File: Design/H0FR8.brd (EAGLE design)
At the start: 34.6 x 30 mm, 45 parts, among them P1 HEXABIT_17.32_NO_P6, Q1 MMBT3904LT1, U1 STM32G0B1CEU6N, U2 T2035H-6GD2PAK_T2550_STM-M, U3 VOT8121AM-VT, U4 TLP184_GR-TPL,SE, X1 XTALL_CSTCE8M00G52

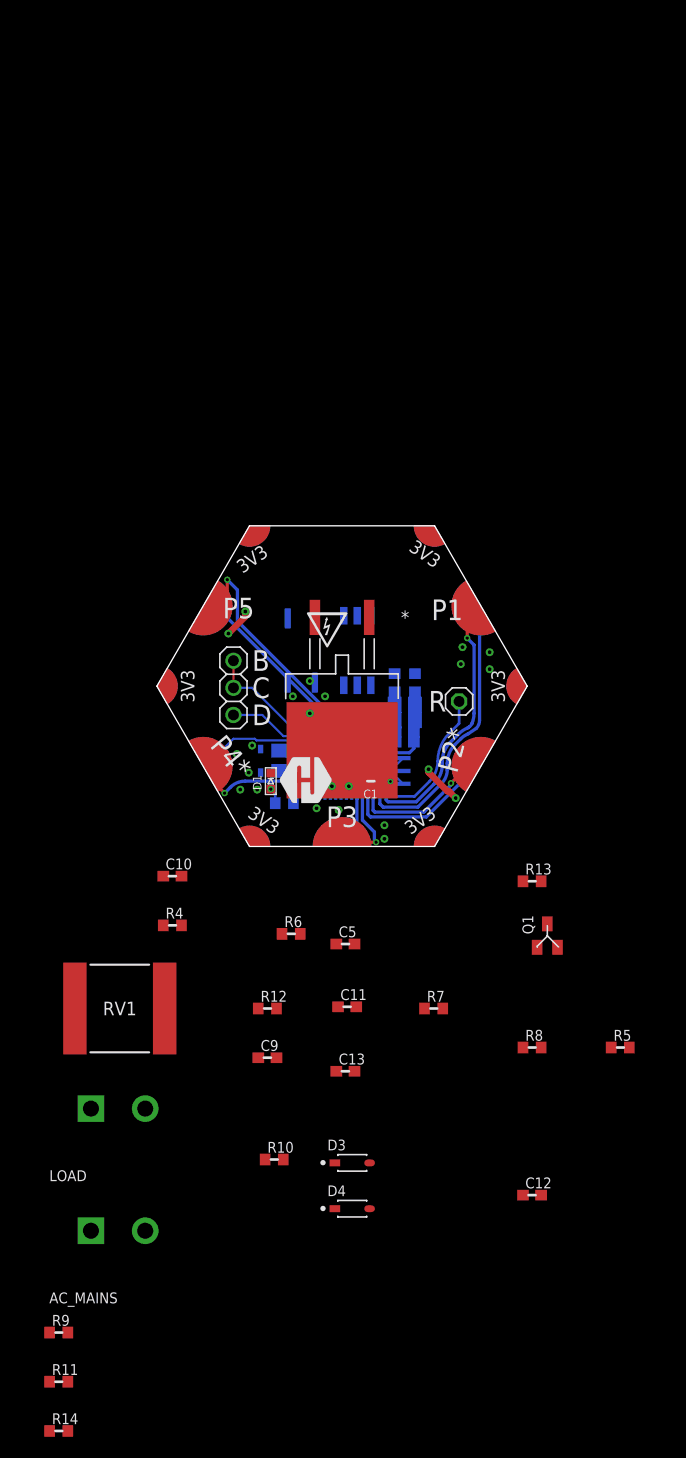
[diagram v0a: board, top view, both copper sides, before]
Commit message: Schematic modification
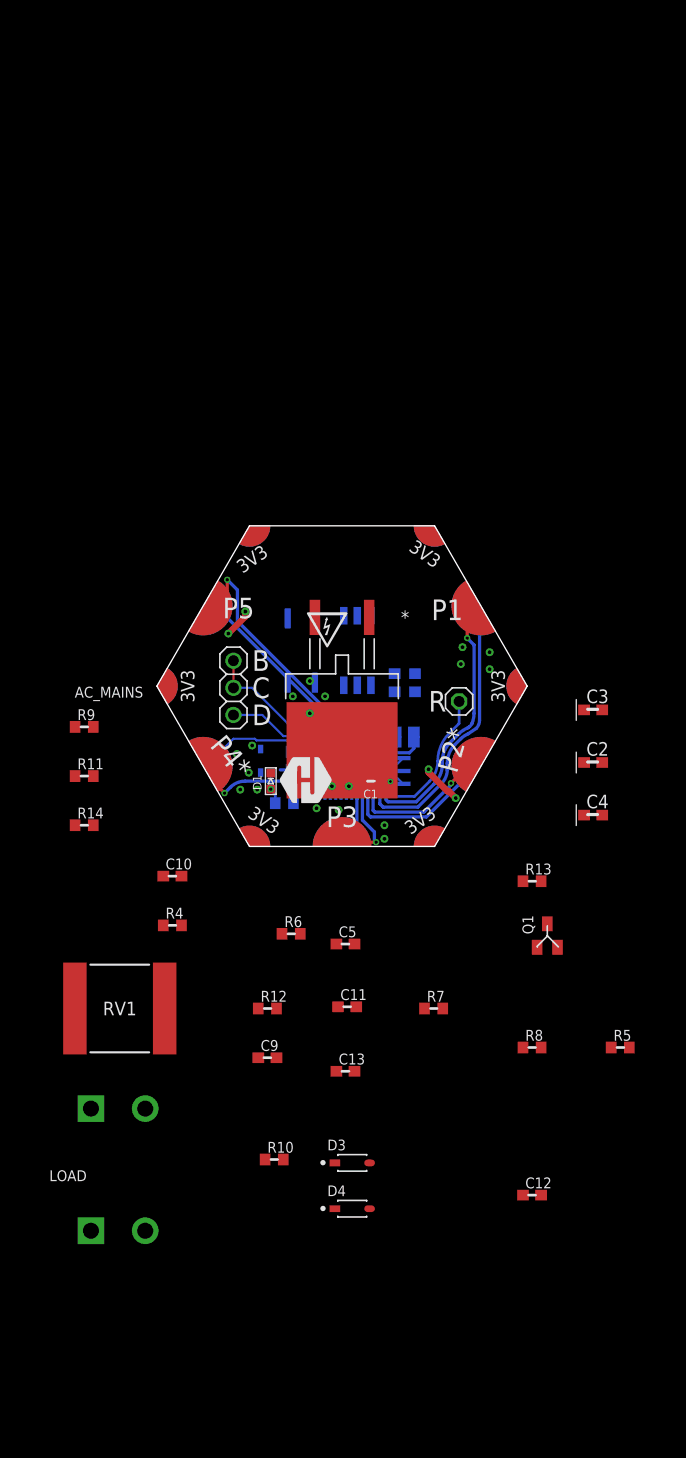
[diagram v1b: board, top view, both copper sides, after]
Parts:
- C2, C3, C4: device HEXABITZ_RCLS:C-0805-POL -> HEXABITZ_RCLS:C-0603-POL
- moved R11 56.7 mm to (-24.1, 6.51)
- moved R14 56.7 mm to (-24.1, 1.91)
- moved R9 56.7 mm to (-24.1, 11.1)
- moved C4 29.8 mm to (23.5, 2.86), flipped to the top, turned to 0 degrees
- moved C2 18.4 mm to (23.5, 7.78), flipped to the top, turned to 0 degrees
- moved C3 17.6 mm to (23.5, 12.7), flipped to the top, turned to 0 degrees

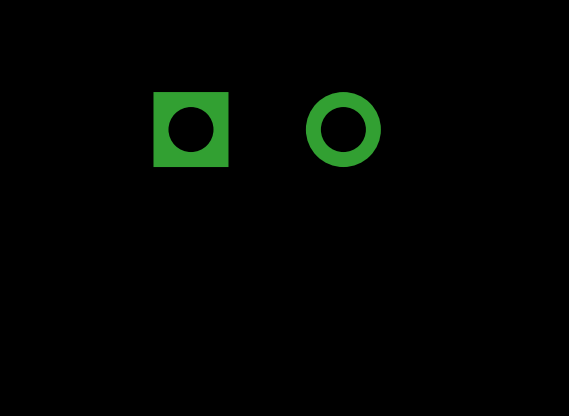
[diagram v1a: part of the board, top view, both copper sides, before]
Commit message: Schematic modification
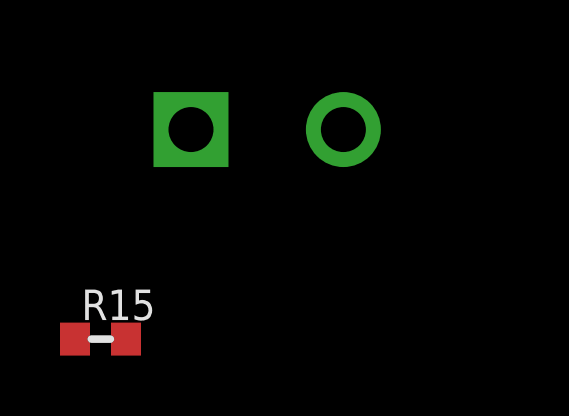
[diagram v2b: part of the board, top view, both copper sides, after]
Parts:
- added R15: 100k, HEXABITZ_RCLS:R-0603
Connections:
- net GND: now also R15.2
- net N$13: now also R15.1
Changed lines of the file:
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@@
 <attribute name="VOLTAGE_RATING" value="25V" x="23.495" y="2.8575" size="1.778" layer="27" display="off"/>
+</element>
+<element name="R15" library="HEXABITZ_RCLS" library_urn="urn:adsk.eagle:library:20064561" package="R-0603" package3d_urn="urn:adsk.eagle:package:1435818/6" value="100k" x="-26.51125" y="-43.02125" smashed="yes">
+<attribute name="MFN" value="Yageo" x="-26.51125" y="-43.02125" size="1.778" layer="27" display="off"/>
+<attribute name="MPN" value="RC0603JR-070RL" x="-26.51125" y="-43.02125" size="1.778" layer="27" display="off"/>
+<attribute name="NAME" x="-27.14625" y="-42.38625" size="1.016" layer="25"/>
+<attribute name="OCTOPART_URL" value="https://octopart.com/crcw06032k40jnea-vishay-40298967" x="-26.51125" y="-43.02125" size="1.778" layer="27" display="off"/>
+<attribute name="RESISTANCE" value="2400.0 Ω" x="-26.51125" y="-43.02125" size="1.778" layer="27" display="off"/>
+<attribute name="TOLERANCE" value="±5%" x="-26.51125" y="-43.02125" size="1.778" layer="27" display="off"/>
+<attribute name="VALUE" x="-27.14625" y="-44.92625" size="1.016" layer="27"/>
 </element>
 </elements>
@@
 <contactref element="U1" pad="30"/>
 <contactref element="C4" pad="2"/>
-<wire x1="1.1675" y1="-21.11375" x2="24.345" y2="2.8575" width="0" layer="19" extent="1-1"/>
+<contactref element="R15" pad="2"/>
+<wire x1="1.1675" y1="-21.11375" x2="-25.66125" y2="-43.02125" width="0" layer="19" extent="1-1"/>
 <wire x1="3.96875" y1="0.635" x2="1.1675" y2="-21.11375" width="0" layer="19" extent="1-1"/>
 <wire x1="3.96875" y1="1.905" x2="3.96875" y2="0.635" width="0" layer="19" extent="1-1"/>
@@
 <wire x1="-16.52" y1="14.9225" x2="-10.63625" y2="19.84375" width="0" layer="19" extent="16-16"/>
 <wire x1="8.26" y1="29.2325" x2="11.27125" y2="18.57375" width="0" layer="19" extent="16-16"/>
-<wire x1="20.15875" y1="-9.51375" x2="8.26" y2="0.6125" width="0" layer="19" extent="1-16"/>
+<wire x1="24.345" y1="2.8575" x2="10.63625" y2="4.445" width="0" layer="19" extent="1-1"/>
+<wire x1="20.15875" y1="-9.51375" x2="24.345" y2="2.8575" width="0" layer="19" extent="1-1"/>
 </signal>
 <signal name="VDD">
@@
 <contactref element="Q1" pad="1"/>
 <contactref element="C5" pad="1"/>
-<wire x1="18.25875" y1="-9.51375" x2="16.93" y2="-18.89125" width="0" layer="19" extent="1-1"/>
-<wire x1="-0.5325" y1="-9.2075" x2="18.25875" y2="-9.51375" width="0" layer="19" extent="1-1"/>
+<contactref element="R15" pad="1"/>
+<wire x1="-0.5325" y1="-9.2075" x2="-27.36125" y2="-43.02125" width="0" layer="19" extent="1-1"/>
+<wire x1="18.25875" y1="-9.51375" x2="-0.5325" y2="-9.2075" width="0" layer="19" extent="1-1"/>
+<wire x1="16.93" y1="-18.89125" x2="18.25875" y2="-9.51375" width="0" layer="19" extent="1-1"/>
 </signal>
 <signal name="N$10">

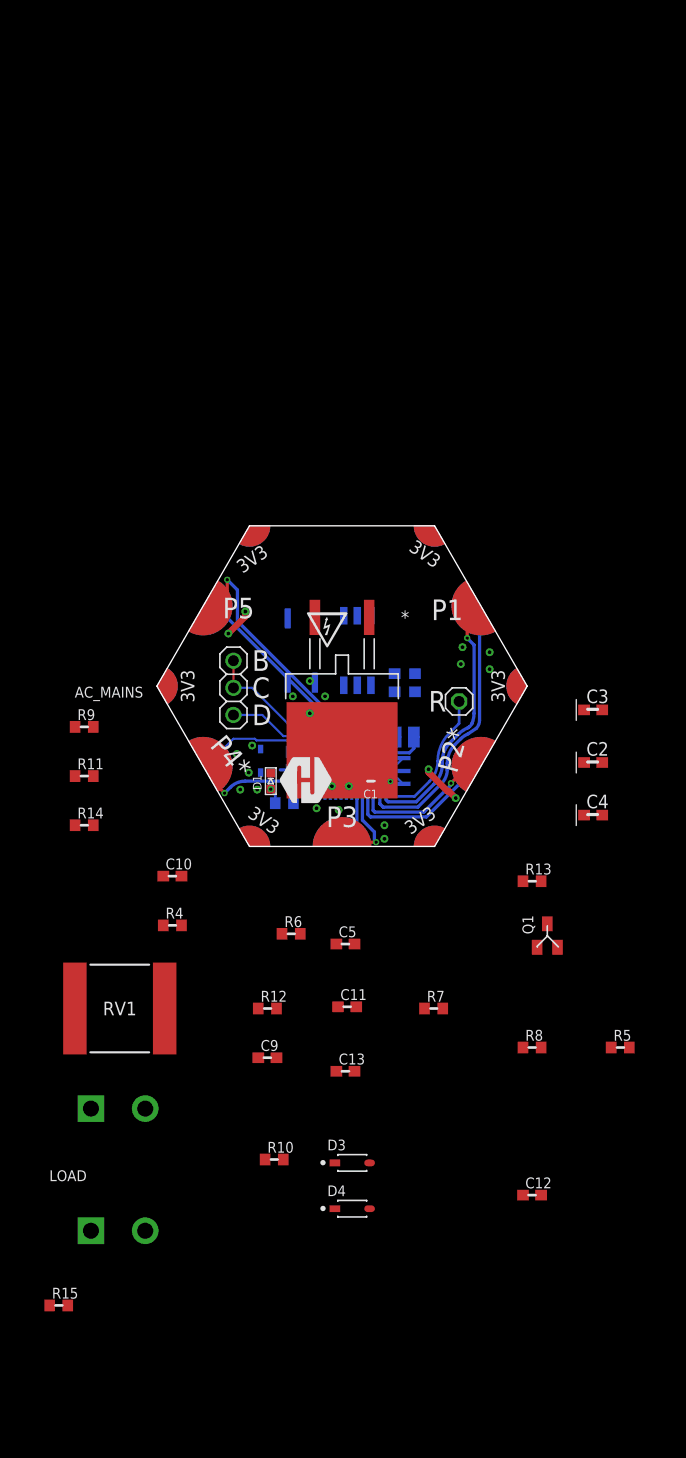
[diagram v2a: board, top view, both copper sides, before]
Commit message: Edit the description
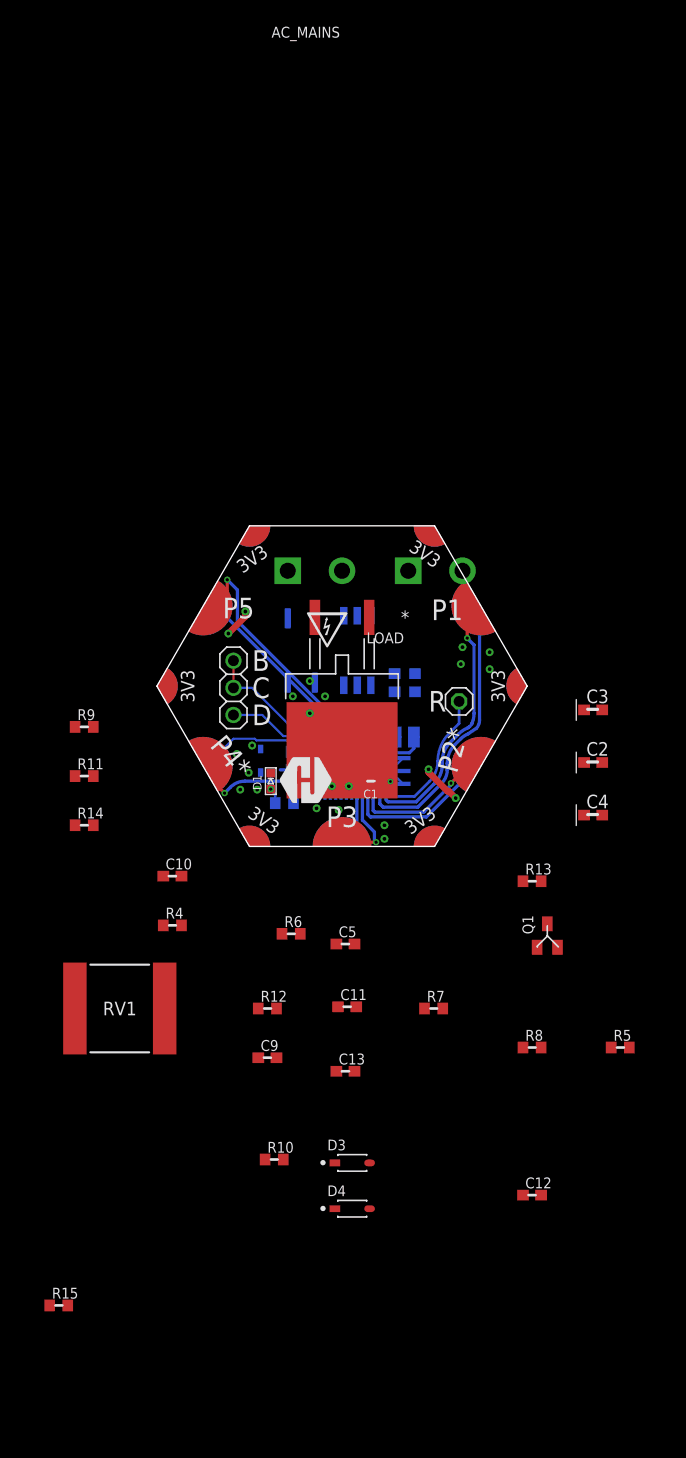
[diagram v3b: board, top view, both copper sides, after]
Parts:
- moved AC_MAINS 64.4 mm to (-2.54, 25.7)
- moved LOAD 58.4 mm to (8.73, 25.7)
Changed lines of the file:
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@@
 <attribute name="VALUE" x="-20.79625" y="-15.24" size="1.27" layer="27" align="center"/>
 </element>
-<element name="LOAD" library="HEXABITZ_CONNECTION_PARTS" library_urn="urn:adsk.eagle:library:20064553" package="1546111-2" package3d_urn="urn:adsk.eagle:package:19666461/4" value="" x="-20.955" y="-24.60625" smashed="yes">
-<attribute name="MFN" value="TE Connectivity" x="-20.955" y="-24.60625" size="1.778" layer="27" display="off"/>
-<attribute name="MPN" value="1546111-2" x="-20.955" y="-24.60625" size="1.778" layer="27" display="off"/>
-<attribute name="NAME" x="-27.395" y="-31.39625" size="1.016" layer="25"/>
-<attribute name="OCTOPART_URL" value="https://octopart.com/1546111-2-te+connectivity-40393355" x="-20.955" y="-24.60625" size="1.778" layer="27" display="off"/>
-<attribute name="VALUE" x="-27.395" y="-32.80625" size="1.016" layer="27"/>
-</element>
-<element name="AC_MAINS" library="HEXABITZ_CONNECTION_PARTS" library_urn="urn:adsk.eagle:library:20064553" package="1546111-2" package3d_urn="urn:adsk.eagle:package:19666461/4" value="" x="-20.955" y="-36.03625" smashed="yes">
-<attribute name="MFN" value="TE Connectivity" x="-20.955" y="-36.03625" size="1.778" layer="27" display="off"/>
-<attribute name="MPN" value="1546111-2" x="-20.955" y="-36.03625" size="1.778" layer="27" display="off"/>
-<attribute name="NAME" x="-25.01375" y="13.8475" size="1.016" layer="25"/>
-<attribute name="OCTOPART_URL" value="https://octopart.com/1546111-2-te+connectivity-40393355" x="-20.955" y="-36.03625" size="1.778" layer="27" display="off"/>
-<attribute name="VALUE" x="-27.395" y="-44.23625" size="1.016" layer="27"/>
+<element name="LOAD" library="HEXABITZ_CONNECTION_PARTS" library_urn="urn:adsk.eagle:library:20064553" package="1546111-2" package3d_urn="urn:adsk.eagle:package:19666461/4" value="" x="8.73125" y="25.7175" smashed="yes">
+<attribute name="MFN" value="TE Connectivity" x="8.73125" y="25.7175" size="1.778" layer="27" display="off"/>
+<attribute name="MPN" value="1546111-2" x="8.73125" y="25.7175" size="1.778" layer="27" display="off"/>
+<attribute name="NAME" x="2.29125" y="18.9275" size="1.016" layer="25"/>
+<attribute name="OCTOPART_URL" value="https://octopart.com/1546111-2-te+connectivity-40393355" x="8.73125" y="25.7175" size="1.778" layer="27" display="off"/>
+<attribute name="VALUE" x="2.29125" y="17.5175" size="1.016" layer="27"/>
+</element>
+<element name="AC_MAINS" library="HEXABITZ_CONNECTION_PARTS" library_urn="urn:adsk.eagle:library:20064553" package="1546111-2" package3d_urn="urn:adsk.eagle:package:19666461/4" value="" x="-2.54" y="25.7175" smashed="yes">
+<attribute name="MFN" value="TE Connectivity" x="-2.54" y="25.7175" size="1.778" layer="27" display="off"/>
+<attribute name="MPN" value="1546111-2" x="-2.54" y="25.7175" size="1.778" layer="27" display="off"/>
+<attribute name="NAME" x="-6.59875" y="75.60125" size="1.016" layer="25"/>
+<attribute name="OCTOPART_URL" value="https://octopart.com/1546111-2-te+connectivity-40393355" x="-2.54" y="25.7175" size="1.778" layer="27" display="off"/>
+<attribute name="VALUE" x="-8.98" y="17.5175" size="1.016" layer="27"/>
 </element>
 <element name="R12" library="HEXABITZ_RCLS" library_urn="urn:adsk.eagle:library:20064561" package="R-0603" package3d_urn="urn:adsk.eagle:package:1435818/6" value="100" x="-6.985" y="-15.24" smashed="yes">
@@
 <contactref element="LOAD" pad="1"/>
 <contactref element="R10" pad="2"/>
-<wire x1="-23.495" y1="-36.03625" x2="-5.5" y2="-29.36875" width="0" layer="19" extent="1-1"/>
-<wire x1="-23.495" y1="-24.60625" x2="-23.495" y2="-36.03625" width="0" layer="19" extent="1-1"/>
+<wire x1="-5.08" y1="25.7175" x2="-5.5" y2="-29.36875" width="0" layer="19" extent="1-1"/>
+<wire x1="6.19125" y1="25.7175" x2="-5.08" y2="25.7175" width="0" layer="19" extent="1-1"/>
 </signal>
 <signal name="AC_MAINS_N">
@@
 <contactref element="C11" pad="2"/>
 <contactref element="R11" pad="2"/>
-<wire x1="-18.415" y1="-36.03625" x2="-23.28" y2="6.50875" width="0" layer="19" extent="1-1"/>
-<wire x1="-6.135" y1="-19.84375" x2="-18.415" y2="-36.03625" width="0" layer="19" extent="1-1"/>
+<wire x1="0" y1="25.7175" x2="-23.28" y2="6.50875" width="0" layer="19" extent="1-1"/>
+<wire x1="-6.135" y1="-19.84375" x2="0" y2="25.7175" width="0" layer="19" extent="1-1"/>
 <wire x1="1.32625" y1="-15.08125" x2="-6.135" y2="-19.84375" width="0" layer="19" extent="1-1"/>
 <wire x1="-16.59625" y1="-15.24" x2="-6.135" y2="-19.84375" width="0" layer="19" extent="1-1"/>
@@
 <contactref element="R13" pad="2"/>
 <wire x1="-6.135" y1="-15.24" x2="18.63" y2="-3.33375" width="0" layer="19" extent="1-1"/>
-<wire x1="-18.415" y1="-24.60625" x2="-6.135" y2="-15.24" width="0" layer="19" extent="1-1"/>
-<wire x1="-24.99625" y1="-15.24" x2="-18.415" y2="-24.60625" width="0" layer="19" extent="1-1"/>
+<wire x1="11.27125" y1="25.7175" x2="-6.135" y2="-15.24" width="0" layer="19" extent="1-1"/>
+<wire x1="-24.99625" y1="-15.24" x2="11.27125" y2="25.7175" width="0" layer="19" extent="1-1"/>
 <wire x1="0" y1="8.92175" x2="-24.99625" y2="-15.24" width="0" layer="19" extent="1-1"/>
 </signal>
